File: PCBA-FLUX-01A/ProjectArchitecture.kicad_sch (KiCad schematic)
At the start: 20 parts, among them J1 Conn_02x05_Odd_Even, J10 Screw_Terminal_01x01, J4 Screw_Terminal_01x01, J5 Screw_Terminal_01x01, J6 Screw_Terminal_01x01, J7 Conn_02x02_Odd_Even, J8 Conn_02x02_Odd_Even, J9 Screw_Terminal_01x01

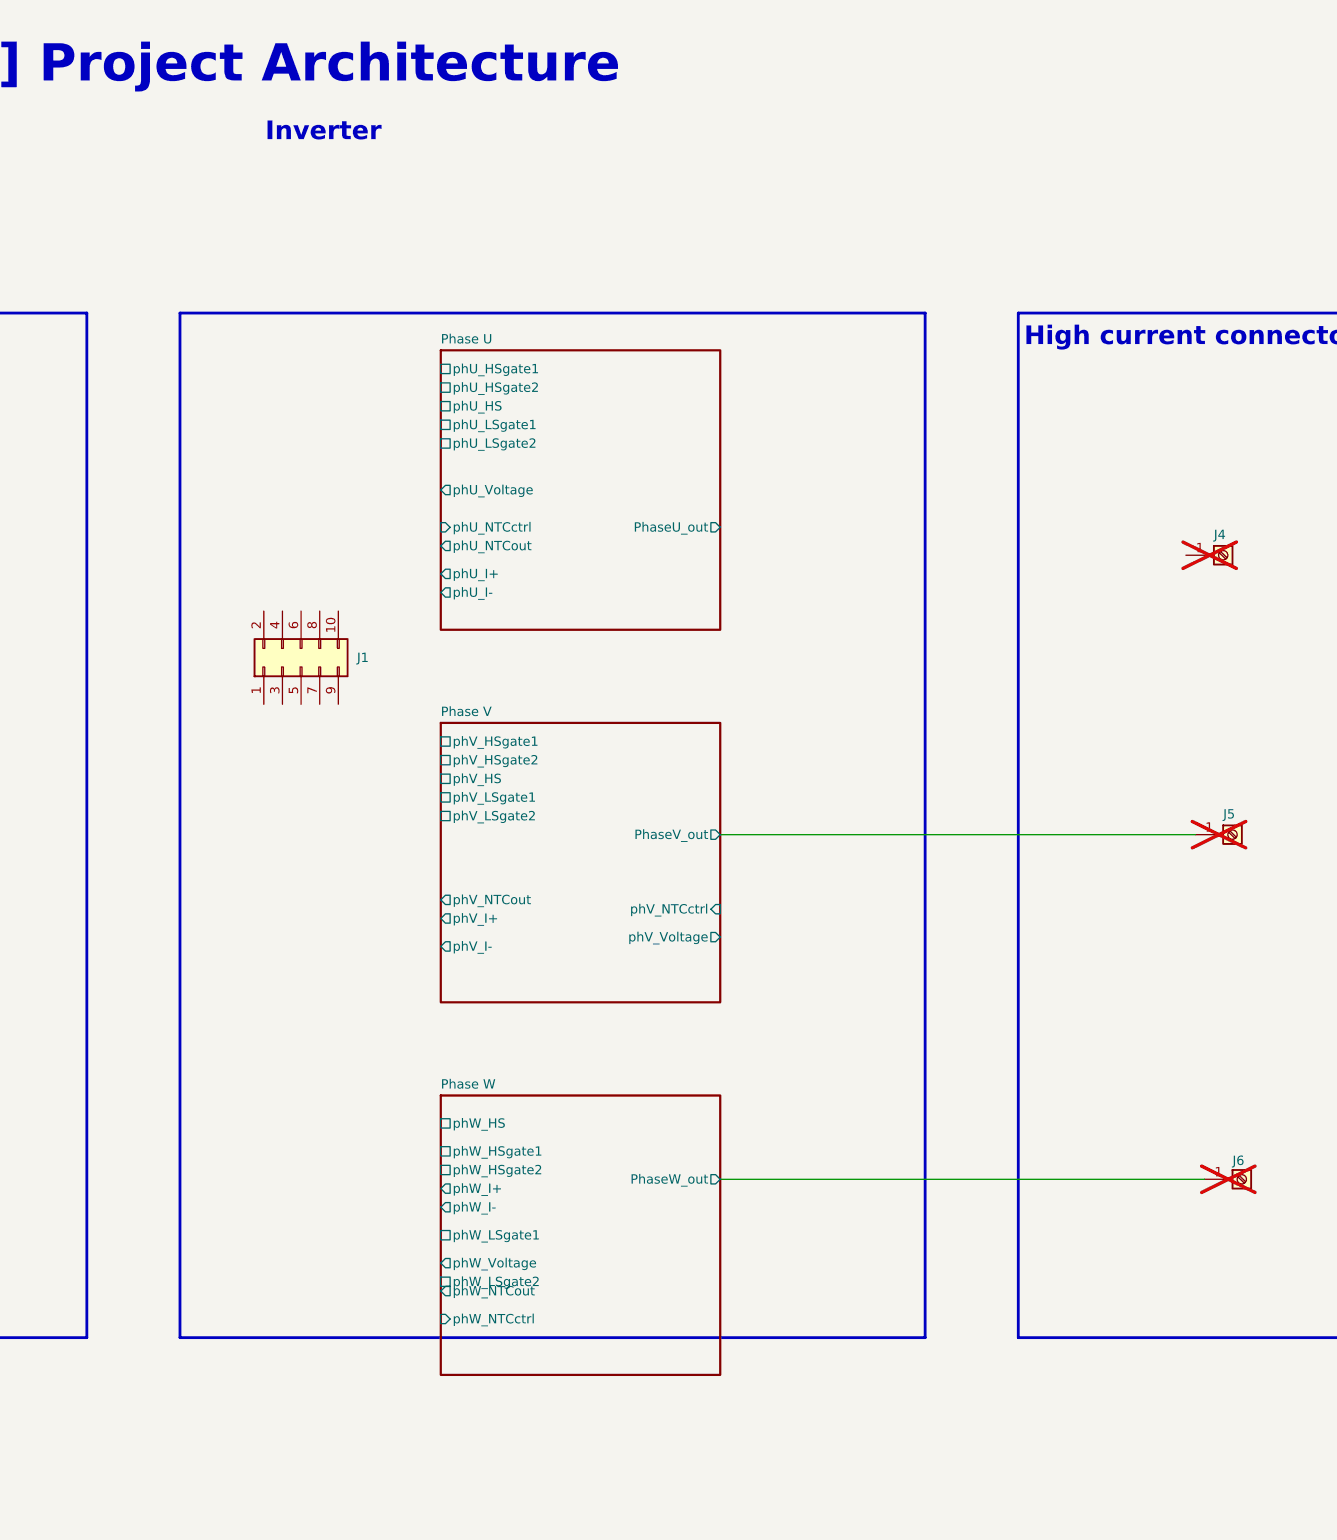
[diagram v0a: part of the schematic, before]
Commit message: :}
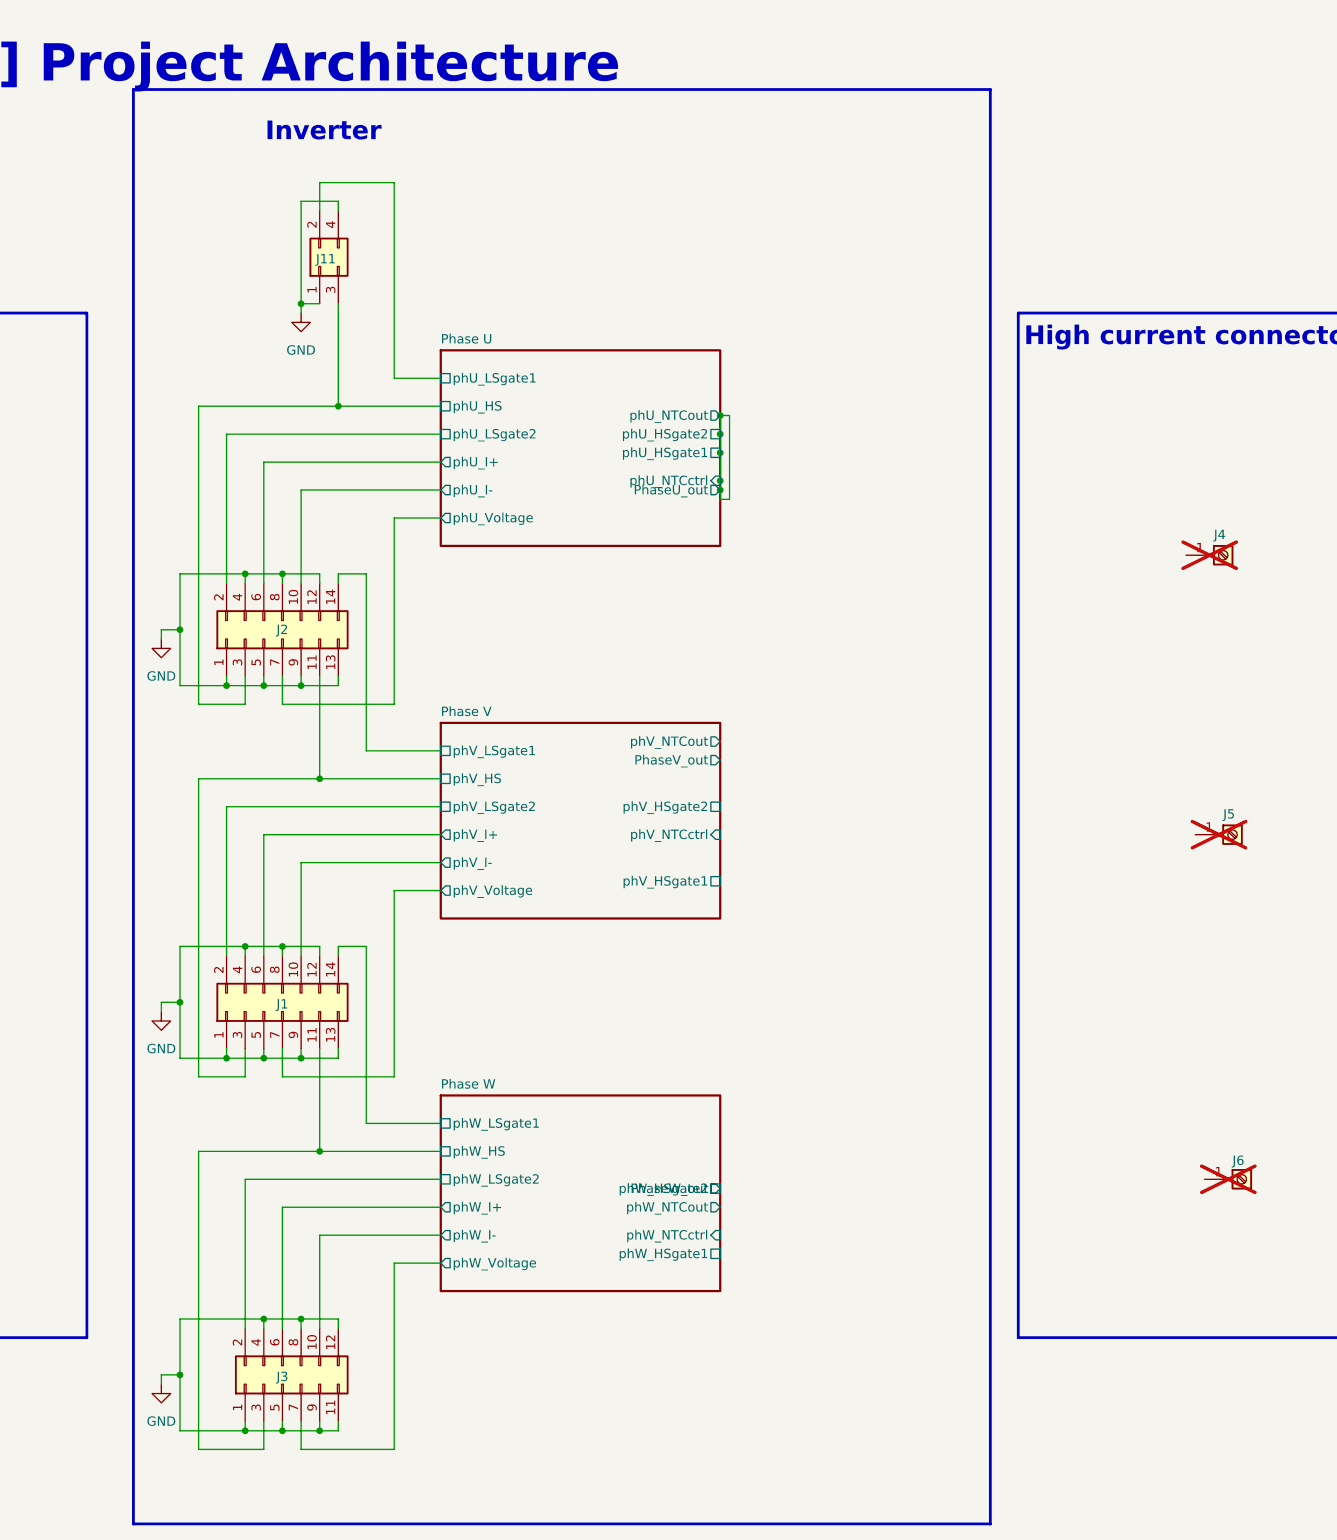
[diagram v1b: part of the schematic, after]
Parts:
- removed J1: Conn_02x05_Odd_Even, symbol Connector_Generic:Conn_02x05_Odd_Even
- added J1, J2: Conn_02x07_Odd_Even, Connector_PinHeader_2.54mm:PinHeader_2x07_P2.54mm_Vertical, symbol Connector_Generic:Conn_02x07_Odd_Even
- added J11: Conn_02x02_Odd_Even, Connector_PinHeader_2.54mm:PinHeader_2x02_P2.54mm_Vertical, symbol Connector_Generic:Conn_02x02_Odd_Even
- added J3: Conn_02x06_Odd_Even, Connector_PinHeader_2.54mm:PinHeader_2x06_P2.54mm_Vertical, symbol Connector_Generic:Conn_02x06_Odd_Even
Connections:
- net GND: now also J1.1 (Pin_1), J1.12 (Pin_12), J1.13 (Pin_13), J1.4 (Pin_4), J1.5 (Pin_5), J1.8 (Pin_8), J1.9 (Pin_9), J11.1 (Pin_1), J11.4 (Pin_4), J2.1 (Pin_1), J2.12 (Pin_12), J2.13 (Pin_13), J2.4 (Pin_4), J2.5 (Pin_5), J2.8 (Pin_8), J2.9 (Pin_9), J3.1 (Pin_1), J3.11 (Pin_11), J3.12 (Pin_12), J3.4 (Pin_4), J3.5 (Pin_5), J3.8 (Pin_8), J3.9 (Pin_9)
- net Phase U/phU_HS: now also J11.3 (Pin_3), J2.3 (Pin_3)
- net Phase U/phU_I+: now also J2.6 (Pin_6)
- net Phase U/phU_I-: now also J2.10 (Pin_10)
- net Phase U/phU_LSgate1: now also J11.2 (Pin_2)
- net Phase U/phU_LSgate2: now also J2.2 (Pin_2)
- net Phase U/phU_Voltage: now also J2.7 (Pin_7)
- net Phase V/PhaseV_out: no longer J5.1 (Pin_1)
- net Phase V/phV_HS: now also J1.3 (Pin_3), J2.11 (Pin_11)
- net Phase V/phV_I+: now also J1.6 (Pin_6)
- net Phase V/phV_I-: now also J1.10 (Pin_10)
- net Phase V/phV_LSgate1: now also J2.14 (Pin_14)
- net Phase V/phV_LSgate2: now also J1.2 (Pin_2)
- net Phase V/phV_Voltage: now also J1.7 (Pin_7)
- net Phase W/PhaseW_out: no longer J6.1 (Pin_1)
- net Phase W/phW_HS: now also J1.11 (Pin_11), J3.3 (Pin_3)
- net Phase W/phW_I+: now also J3.6 (Pin_6)
- net Phase W/phW_I-: now also J3.10 (Pin_10)
- net Phase W/phW_LSgate1: now also J1.14 (Pin_14)
- net Phase W/phW_LSgate2: now also J3.2 (Pin_2)
- net Phase W/phW_Voltage: now also J3.7 (Pin_7)
